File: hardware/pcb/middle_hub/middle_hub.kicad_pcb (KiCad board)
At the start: 2 copper layers, 19 x 50.5 mm, 26 parts, among them J1 USB_A, J2 FH34SRJ-12S-0.5SH, J3 FH34SRJ-12S-0.5SH, J4 Conn_01x05, SW1 RotaryEncoder_Switch, U2 AP2112K-3.3, U3 NC7SB3157P6X, U4 NC7SB3157P6X, U5 PRTR5V0U2X

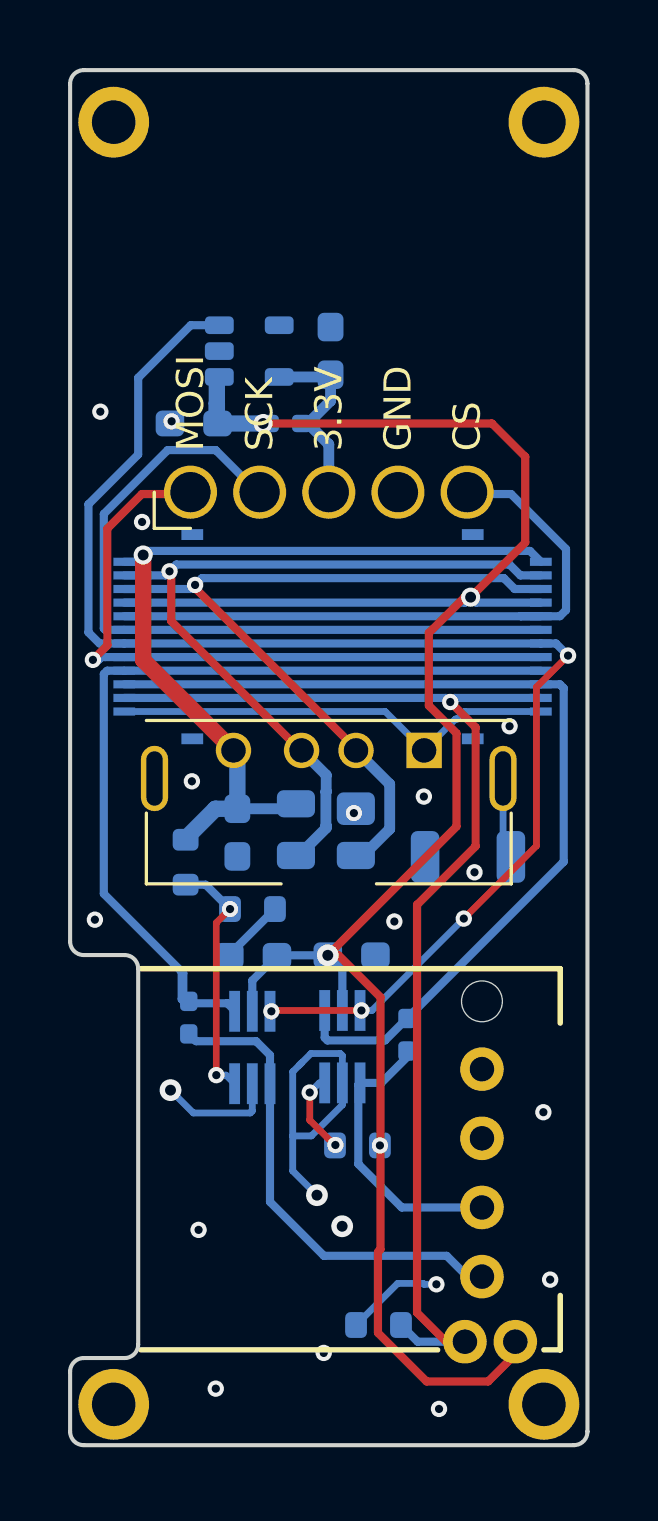
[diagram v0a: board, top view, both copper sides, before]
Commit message: temp
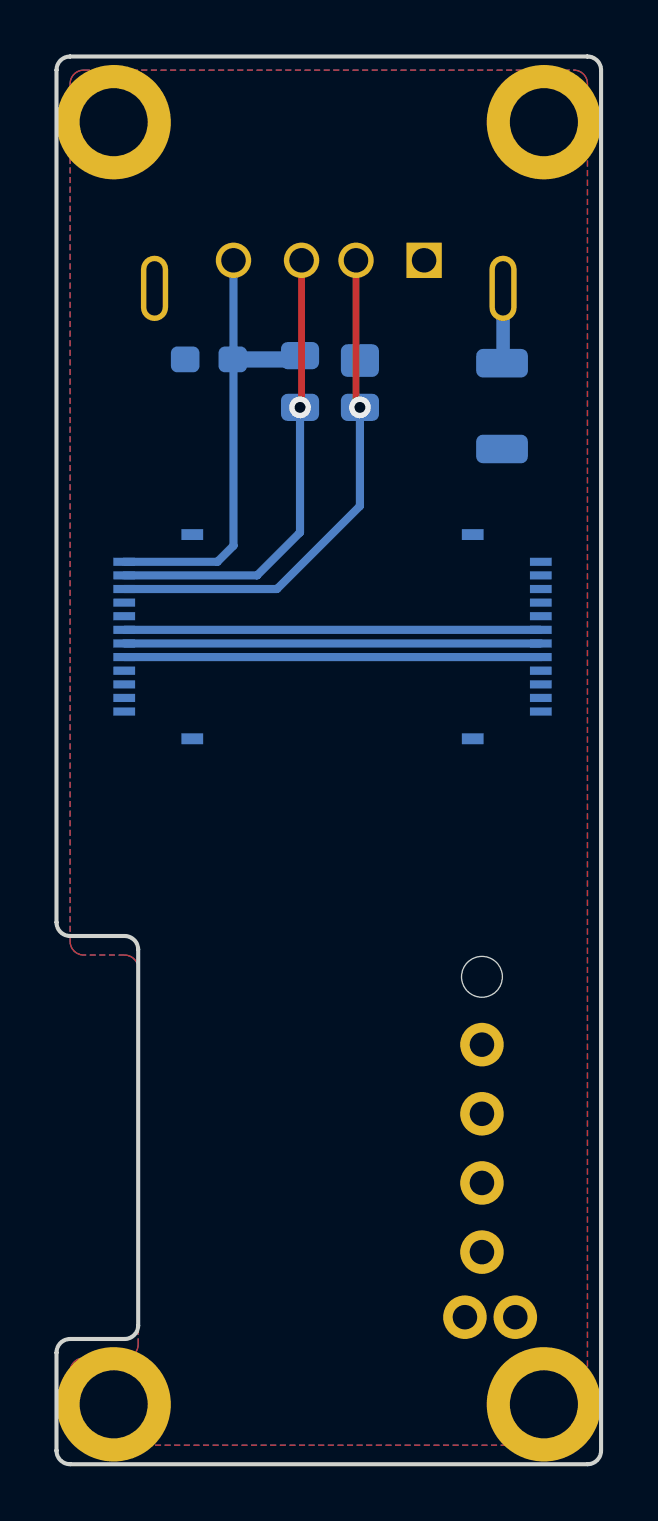
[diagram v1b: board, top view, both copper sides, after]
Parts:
- removed C2, C3, C6, C7: C_Small, PCM_Capacitor_SMD_AKL:C_0603_1608Metric_Pad1.05x0.95mm
- removed J4: Conn_01x05, ec_parts:NiceView_PinHeader_1x05_P2.54mm
- removed R1, R2, R3: 0, PCM_Resistor_SMD_AKL:R_0402_1005Metric_Pad0.72x0.64mm_HandSolder
- removed R4, R5: 10k, PCM_Resistor_SMD_AKL:R_0603_1608Metric
- removed R6: 5.1k, PCM_Resistor_SMD_AKL:R_0603_1608Metric
- removed R7: 1k, PCM_Resistor_SMD_AKL:R_0603_1608Metric
- removed U2: AP2112K-3.3, PCM_Package_TO_SOT_SMD_AKL:SOT-23-5
- removed U3, U4: NC7SB3157P6X, PCM_Package_TO_SOT_SMD_AKL:SOT-363_SC-70-6_Handsoldering
- moved J1 18.0 mm to (200.0, 54.5)
- moved C1 17.4 mm to (195.6, 57.6), turned to 0 degrees
- moved L1 16.6 mm to (206.4, 59.3), turned to 90 degrees
- moved U5 16.5 mm to (200.0, 58.4)
- moved SW1 0.90 mm to (200.0, 86.6)
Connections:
- J2 pad 2: ENC_S1 -> unconnected-(J2-Pin_2-Pad2)
- J2 pad 3: INPUT_B -> unconnected-(J2-Pin_3-Pad3)
- J2 pad 4: INPUT_A -> unconnected-(J2-Pin_4-Pad4)
- J2 pad 5: SPI_MOSI -> ENC_S1
- J2 pad 6: EXT_POWER -> INPUT_B
- J2 pad 7: SPI_SCK  -> INPUT_A
- J2 pad 8: SPI_CS   -> unconnected-(J2-Pin_8-Pad8)
- J2 pad 9: +3V3 -> unconnected-(J2-Pin_9-Pad9)
- J3 pad 1: VBUS -> unconnected-(J3-Pin_1-Pad1)
- J3 pad 10: INPUT_B -> unconnected-(J3-Pin_10-Pad10)
- J3 pad 11: ENC_S1 -> unconnected-(J3-Pin_11-Pad11)
- J3 pad 2: /DM4 -> unconnected-(J3-Pin_2-Pad2)
- J3 pad 3: /DP4 -> unconnected-(J3-Pin_3-Pad3)
- J3 pad 4: +3V3 -> unconnected-(J3-Pin_4-Pad4)
- J3 pad 5: SPI_CS   -> unconnected-(J3-Pin_5-Pad5)
- J3 pad 6: SPI_SCK  -> INPUT_A
- J3 pad 7: EXT_POWER -> INPUT_B
- J3 pad 8: SPI_MOSI -> ENC_S1
- J3 pad 9: INPUT_A -> unconnected-(J3-Pin_9-Pad9)
- SW1 pad S1: +3V3 -> GND
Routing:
- net +3V3: track 79.3 -> 0.00 mm, vias 4 -> 0
- net EXT_POWER: track 51.5 -> 0.00 mm, vias 4 -> 0
- net GND: track 38.1 -> 0.00 mm, vias 20 -> 0
- net ENC_S1: track 43.9 -> 15.3 mm, vias 1 -> 0
- net SPI_SCK : track 27.6 -> 0.00 mm
- net SPI_MOSI: track 25.1 -> 0.00 mm, vias 1 -> 0
- net SPI_CS  : track 23.8 -> 0.00 mm
- net INPUT_B: track 35.1 -> 15.3 mm
- net INPUT_A: track 32.4 -> 15.3 mm
- net ENC_A : track 17.1 -> 0.00 mm
- net VBUS: track 30.9 -> 17.1 mm, vias 1 -> 0
- net /DM4: track 28.9 -> 17.1 mm
- net ENC_B : track 10.3 -> 0.00 mm
- net /DP4: track 28.8 -> 19.0 mm
- net VBUS_DEC: track 9.16 -> 0.00 mm, vias 2 -> 0
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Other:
- board size 19 x 50.5 mm -> 20 x 51.7 mm
